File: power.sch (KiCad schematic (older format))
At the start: 66 parts, among them SW7 JS202011SCQN, U1 ICE40HX4K-TQ144, U10 MAX40200AUK, U12 TPS562201, U15 MAX40200AUK, U21 MAX40200AUK, U6 TLV62568APDRLR, U7 TLV62568APDRLR

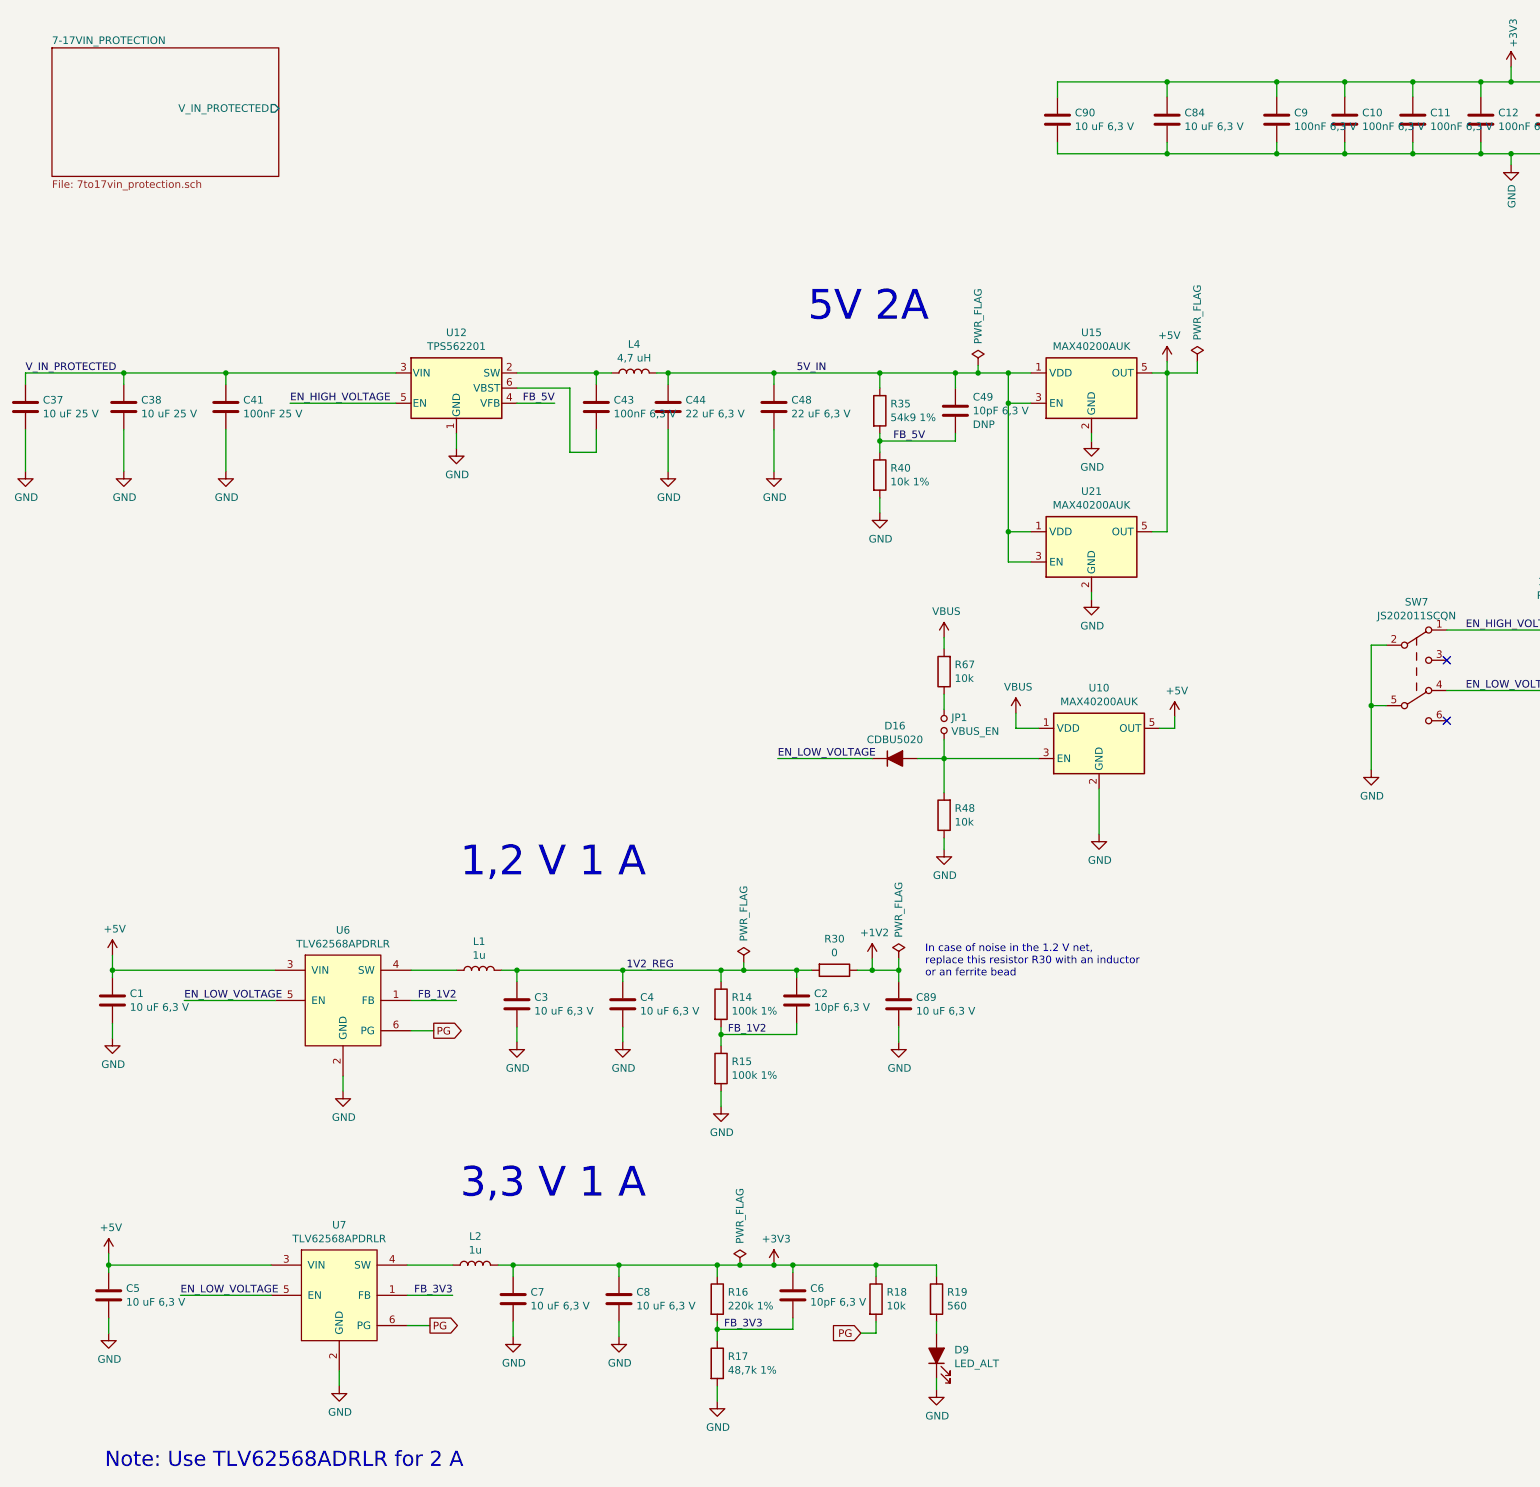
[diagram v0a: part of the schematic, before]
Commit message: Voltage Regulators
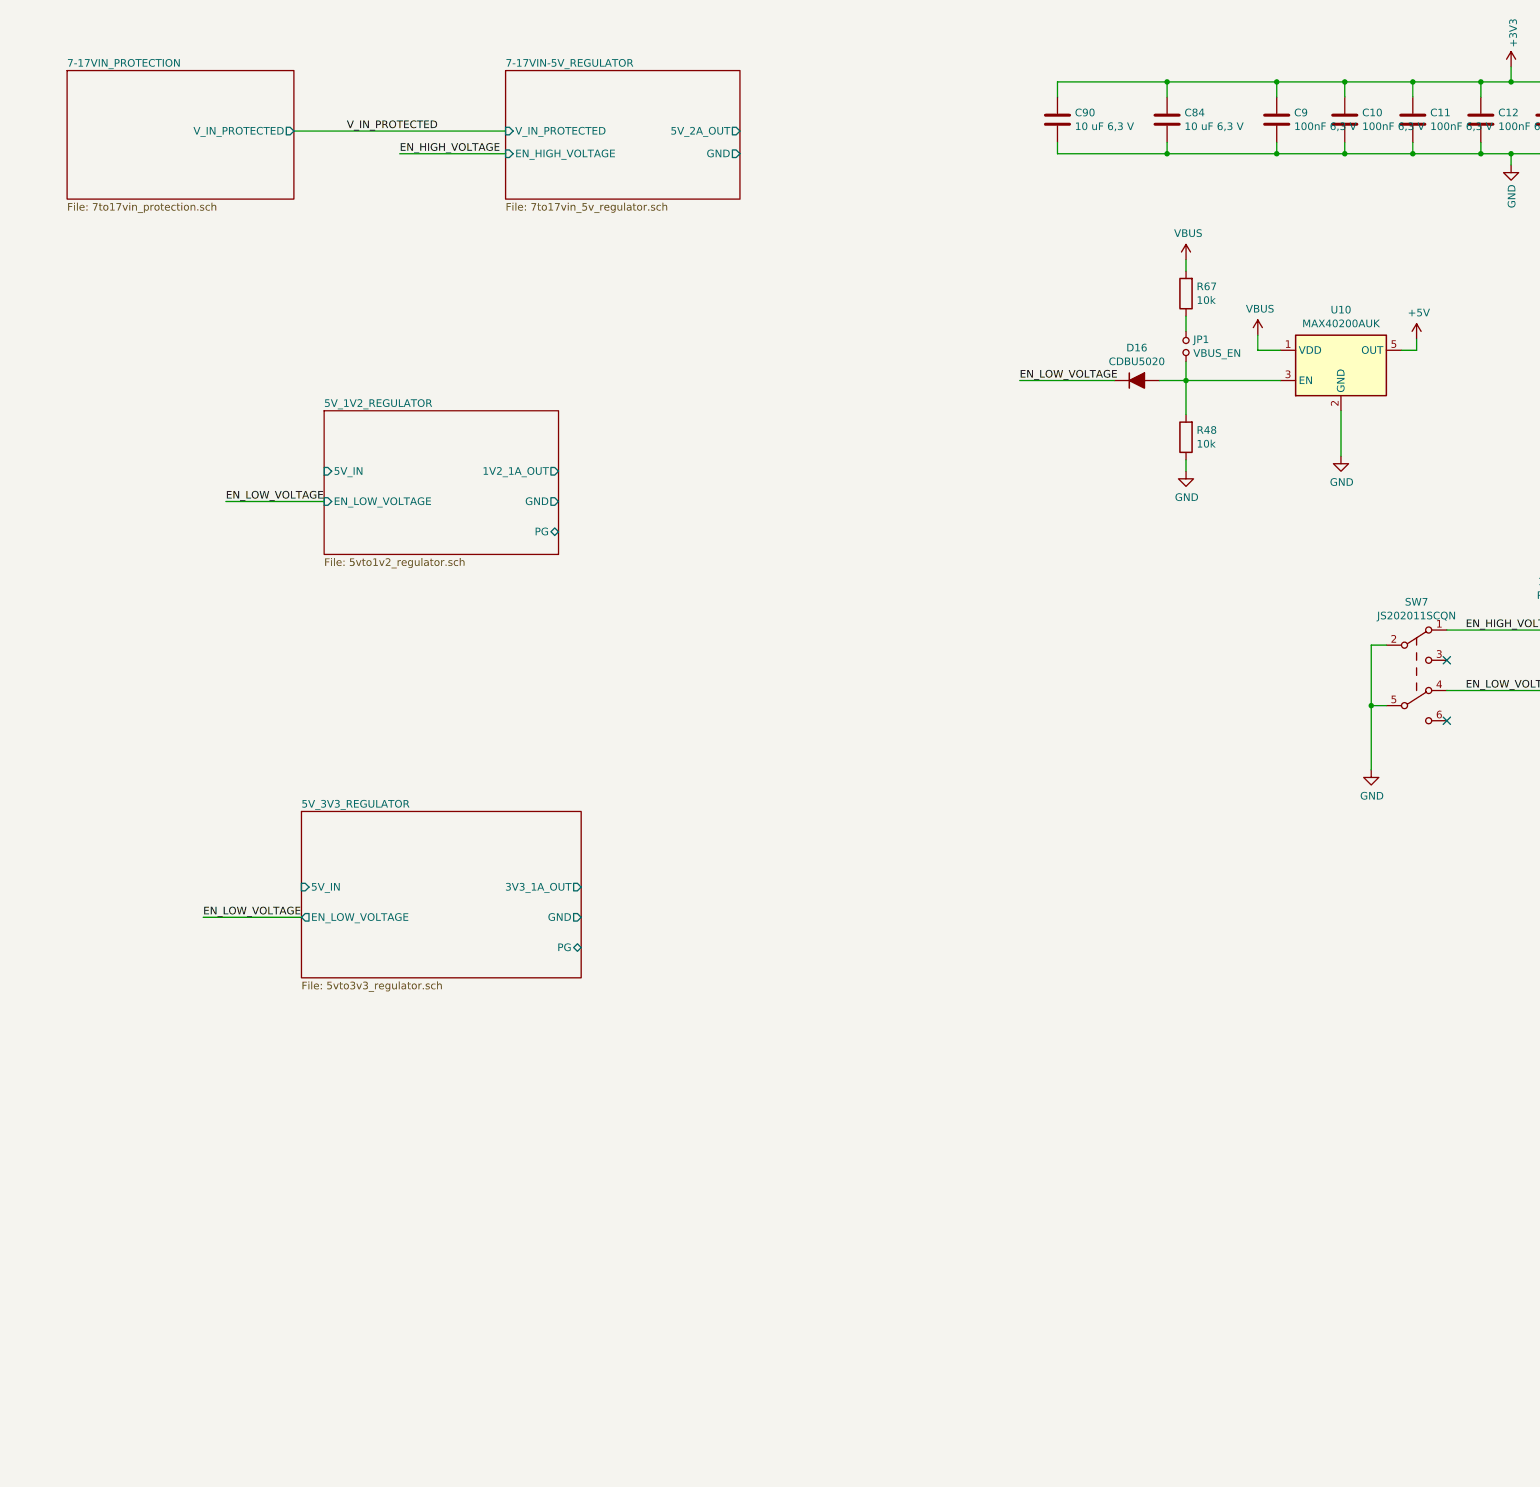
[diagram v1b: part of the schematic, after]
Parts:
- removed C1, C3, C4, C5, C7, C8, C89: 10 uF 6,3 V, Capacitor_SMD:C_0603_1608Metric, symbol Device:C
- removed C2, C49, C6: 10pF 6,3 V, Capacitor_SMD:C_0603_1608Metric, symbol Device:C
- removed C37, C38: 10 uF 25 V, Capacitor_SMD:C_0805_2012Metric, symbol Device:C
- removed C41: 100nF 25 V, Capacitor_SMD:C_0603_1608Metric, symbol Device:C
- removed C43: 100nF 6,3 V, Capacitor_SMD:C_0603_1608Metric, symbol Device:C
- removed C44, C48: 22 uF 6,3 V, Capacitor_SMD:C_0603_1608Metric, symbol Device:C
- removed D9: LED_ALT, LED_SMD:LED_0603_1608Metric, symbol Device:LED_ALT
- removed L1, L2: 1u, footprints:L_1008_2520Metric_2.5x2mm_footprint, symbol Device:L
- removed L4: 4,7 uH, Inductor_SMD:L_Taiyo-Yuden_NR-50xx, symbol Device:L
- removed R14, R15: 100k 1%, Resistor_SMD:R_0603_1608Metric, symbol Device:R
- removed R16: 220k 1%, Resistor_SMD:R_0603_1608Metric, symbol Device:R
- removed R17: 48,7k 1%, Resistor_SMD:R_0603_1608Metric, symbol Device:R
- removed R18: 10k, Resistor_SMD:R_0603_1608Metric, symbol Device:R
- removed R19: 560, Resistor_SMD:R_0603_1608Metric, symbol Device:R
- removed R30: 0, Resistor_SMD:R_0805_2012Metric, symbol Device:R
- removed R35: 54k9 1%, Resistor_SMD:R_0603_1608Metric, symbol Device:R
- removed R40: 10k 1%, Resistor_SMD:R_0603_1608Metric, symbol Device:R
- removed U12: TPS562201, Package_TO_SOT_SMD:SOT-23-6, symbol Regulator_Switching:TPS562200
- removed U15, U21: MAX40200AUK, Package_TO_SOT_SMD:SOT-23-5, symbol Analog_Switch:MAX40200AUK
- removed U6, U7: TLV62568APDRLR, footprints:Texas_DRL_SOT-563_1.6x1.6mm_0.5mm-pitch_footprint, symbol TLV62568APDRLR:TLV62568APDRLR
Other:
- note removed: "1,2 V 1 A"
- note removed: "3,3 V 1 A"
- note removed: "5V 2A"
- note removed: "In case of noise in the 1.2 V net,\nreplace this resistor R30 with an inductor\nor an ferrite bead"
- note removed: "Note: Use TLV62568ADRLR for 2 A"
- moved on the sheet: D16, JP1, R48, R67, U10
